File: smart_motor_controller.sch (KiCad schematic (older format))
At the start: 42 parts, among them J10 USB_B_Micro, J101 Breakout, J102 I2C_CONN, J103 CAN_CONN, J104 Debug, J9 Input 12V, Q101 FDD6685, SW102 SW_NRST, SW103 SW_NRST, U2 STM32F405RGT6, U3 USBLC6-2SC6

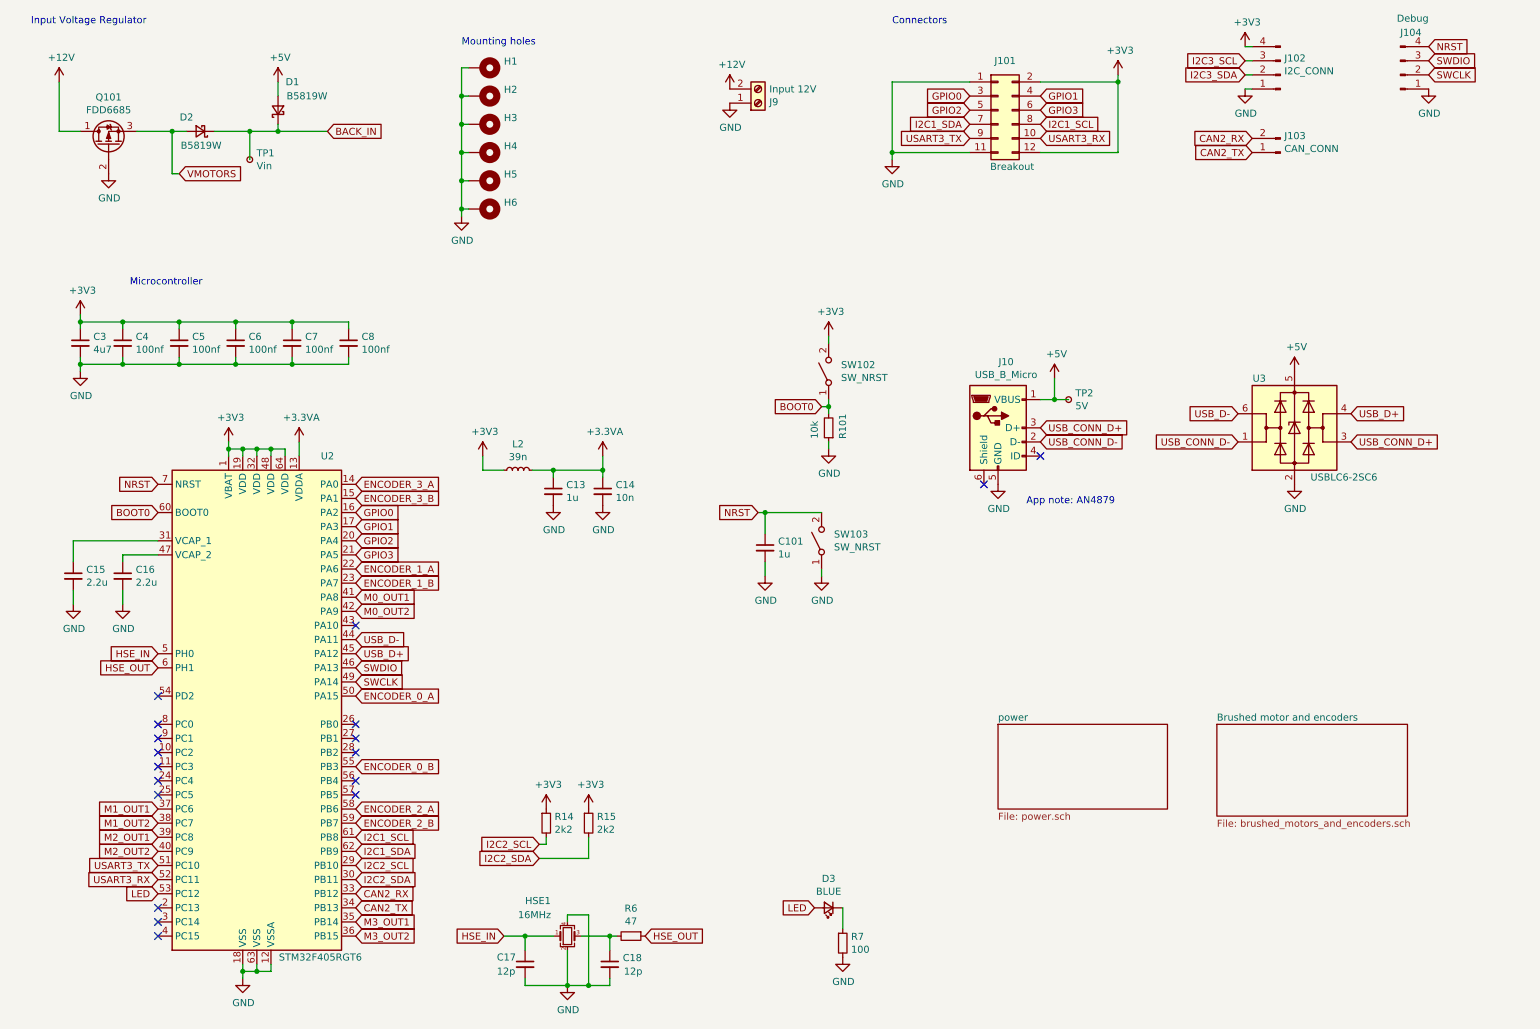
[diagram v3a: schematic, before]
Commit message: Additional changes
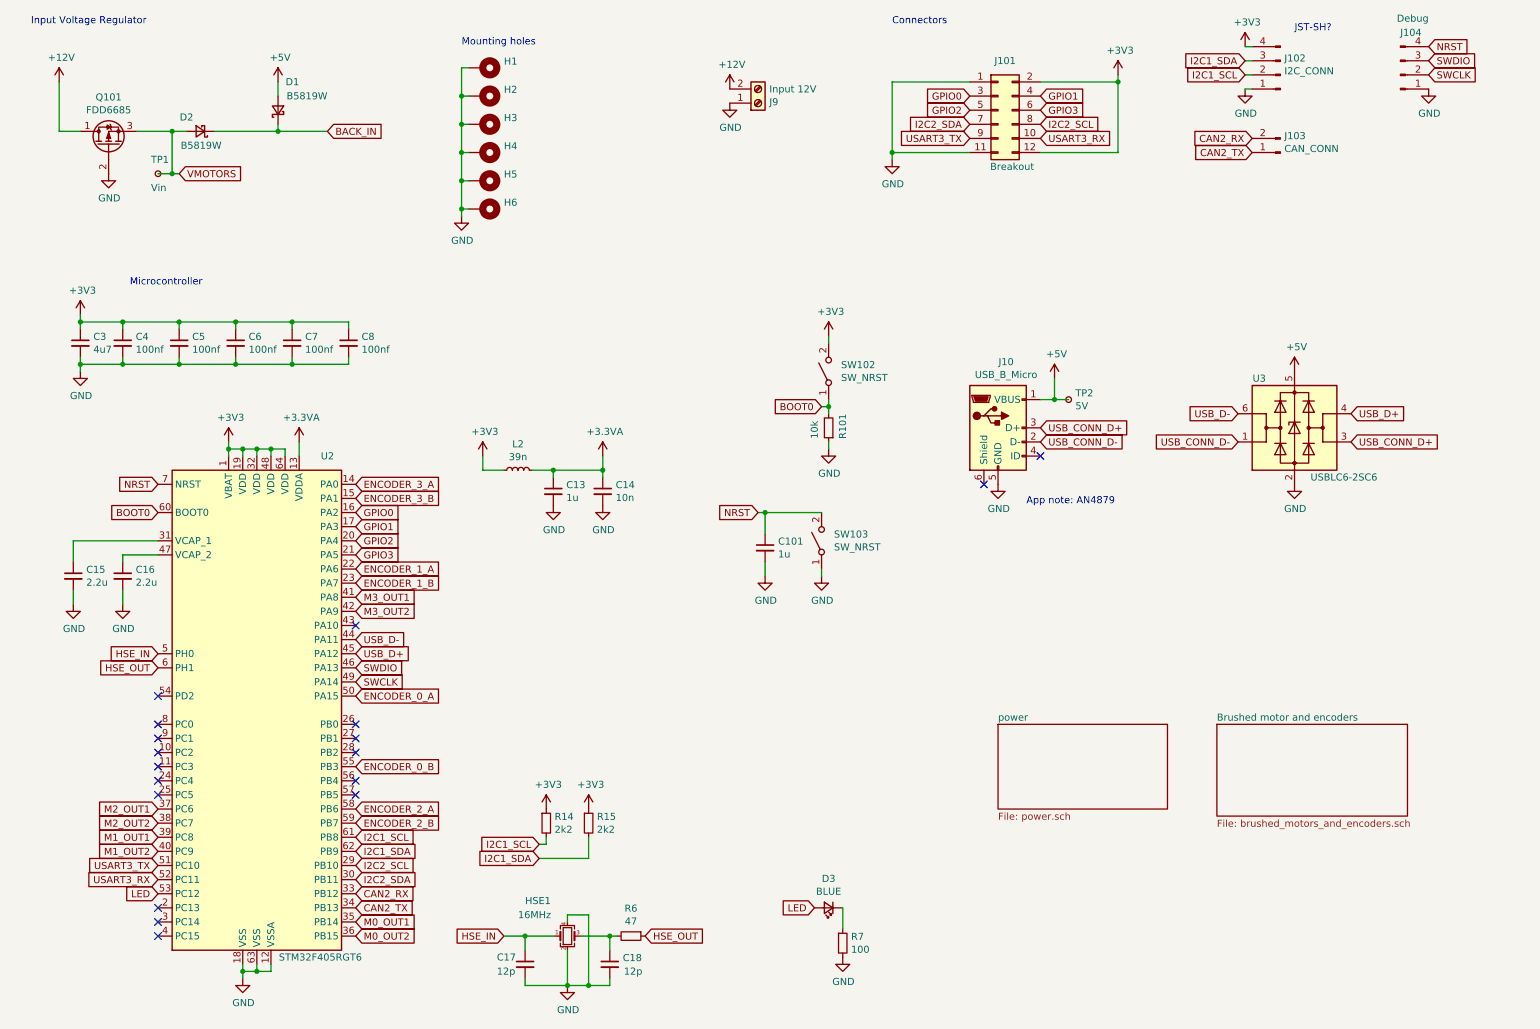
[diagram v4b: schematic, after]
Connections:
- net I2C3_SCL is gone; now on net I2C1_SDA: J102.3 (Pin_3)
- net I2C3_SDA is gone; now on net I2C1_SCL: J102.2 (Pin_2)
- net BACK_IN: no longer TP1.1
- net I2C1_SCL: now also R14.2; no longer J101.8 (Pin_8)
- net I2C1_SDA: now also R15.2; no longer J101.7 (Pin_7)
- net I2C2_SCL: now also J101.8 (Pin_8); no longer R14.2
- net I2C2_SDA: now also J101.7 (Pin_7); no longer R15.2
- net M0_OUT1: now also U2.35 (PB14); no longer U2.41 (PA8)
- net M0_OUT2: now also U2.36 (PB15); no longer U2.42 (PA9)
- net M1_OUT1: now also U2.39 (PC8); no longer U2.37 (PC6)
- net M1_OUT2: now also U2.40 (PC9); no longer U2.38 (PC7)
- net M2_OUT1: now also U2.37 (PC6); no longer U2.39 (PC8)
- net M2_OUT2: now also U2.38 (PC7); no longer U2.40 (PC9)
- net M3_OUT1: now also U2.41 (PA8); no longer U2.35 (PB14)
- net M3_OUT2: now also U2.42 (PA9); no longer U2.36 (PB15)
- net VMOTORS: now also TP1.1
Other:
- note added: "JST-SH?"
- moved on the sheet: TP1
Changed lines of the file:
@@
 Text Notes 1300 2500 0    50   ~ 0
 Microcontroller
-Text GLabel 7750 1350 2    50   Input ~ 0
+Text GLabel 9200 1000 0    50   Input ~ 0
 I2C1_SCL
-Text GLabel 7250 1350 0    50   Input ~ 0
+Text GLabel 9200 900  0    50   Input ~ 0
 I2C1_SDA
 $Comp
@@
 $EndComp
 NoConn ~ 2900 5800
+Text GLabel 2900 7000 2    50   Input ~ 0
+M0_OUT1
+Text GLabel 2900 7100 2    50   Input ~ 0
+M0_OUT2
+Text GLabel 1500 6400 0    50   Input ~ 0
+M1_OUT1
+Text GLabel 1500 6500 0    50   Input ~ 0
+M1_OUT2
+Text GLabel 1500 6200 0    50   Input ~ 0
+M2_OUT1
+Text GLabel 1500 6300 0    50   Input ~ 0
+M2_OUT2
 Text GLabel 2900 4700 2    50   Input ~ 0
-M0_OUT1
+M3_OUT1
 Text GLabel 2900 4800 2    50   Input ~ 0
-M0_OUT2
-Text GLabel 1500 6200 0    50   Input ~ 0
-M1_OUT1
-Text GLabel 1500 6300 0    50   Input ~ 0
-M1_OUT2
-Text GLabel 1500 6400 0    50   Input ~ 0
-M2_OUT1
-Text GLabel 1500 6500 0    50   Input ~ 0
-M2_OUT2
-Text GLabel 2900 7000 2    50   Input ~ 0
-M3_OUT1
-Text GLabel 2900 7100 2    50   Input ~ 0
 M3_OUT2
 NoConn ~ 2900 4900
@@
 Text GLabel 9250 1550 0    50   Input ~ 0
 CAN2_TX
-Text GLabel 9200 900  0    50   Input ~ 0
-I2C3_SCL
-Text GLabel 9200 1000 0    50   Input ~ 0
-I2C3_SDA
+Text GLabel 7750 1350 2    50   Input ~ 0
+I2C2_SCL
+Text GLabel 7250 1350 0    50   Input ~ 0
+I2C2_SDA
 $Comp
 L power:+3V3 #PWR0104
@@
 	4200 6450 4250 6450
 Text GLabel 4200 6550 0    50   Input ~ 0
-I2C2_SDA
+I2C1_SDA
 Text GLabel 4200 6450 0    50   Input ~ 0
-I2C2_SCL
+I2C1_SCL
 $Comp
 L Device:R_Small R15
@@
 L Connector:TestPoint_Small TP1
 U 1 1 604A4E02
-P 2150 1600
-F 0 "TP1" H 2198 1646 50  0000 L CNN
-F 1 "Vin" H 2198 1555 50  0000 L CNN
-F 2 "TestPoint:TestPoint_Pad_D1.5mm" H 2350 1600 50  0001 C CNN
-F 3 "~" H 2350 1600 50  0001 C CNN
-	1    2150 1600
-	1    0    0    -1
-$EndComp
-Wire Wire Line
-	1900 1400 2150 1400
+P 1500 1700
+F 0 "TP1" H 1450 1800 50  0000 L CNN
+F 1 "Vin" H 1450 1600 50  0000 L CNN
+F 2 "TestPoint:TestPoint_Pad_D1.5mm" H 1700 1700 50  0001 C CNN
+F 3 "~" H 1700 1700 50  0001 C CNN
+	1    1500 1700
+	1    0    0    -1
+$EndComp
 Connection ~ 2350 1400
-Wire Wire Line
-	2150 1600 2150 1400
-Connection ~ 2150 1400
-Wire Wire Line
-	2150 1400 2350 1400
 Wire Wire Line
 	1350 1400 1600 1400
@@
 	1    0    0    -1
 $EndComp
-Text GLabel 2900 5900 2    50   Input ~ 0
-ENCODER_0_B
-Text GLabel 2900 5400 2    50   Input ~ 0
-ENCODER_0_A
-Text GLabel 2900 4600 2    50   Input ~ 0
-ENCODER_1_B
-Text GLabel 2900 6300 2    50   Input ~ 0
-ENCODER_2_B
-Text GLabel 2900 6200 2    50   Input ~ 0
-ENCODER_2_A
-Text GLabel 2900 4000 2    50   Input ~ 0
-ENCODER_3_B
-Text GLabel 2900 3900 2    50   Input ~ 0
-ENCODER_3_A
 Text GLabel 1500 6600 0    50   Input ~ 0
 USART3_TX
 Text GLabel 1500 6700 0    50   Input ~ 0
 USART3_RX
-Text GLabel 2900 4500 2    50   Input ~ 0
-ENCODER_1_A
 NoConn ~ 2900 6000
 NoConn ~ 2900 6100
@@
 Text GLabel 10500 900  2    50   Input ~ 0
 SWDIO
+Text GLabel 2900 6200 2    50   Input ~ 0
+ENCODER_2_A
+Text GLabel 2900 6300 2    50   Input ~ 0
+ENCODER_2_B
+Text GLabel 2900 4500 2    50   Input ~ 0
+ENCODER_1_A
+Text GLabel 2900 4600 2    50   Input ~ 0
+ENCODER_1_B
+Text GLabel 2900 4000 2    50   Input ~ 0
+ENCODER_3_B
+Text GLabel 2900 3900 2    50   Input ~ 0
+ENCODER_3_A
+Text GLabel 2900 5400 2    50   Input ~ 0
+ENCODER_0_A
+Text GLabel 2900 5900 2    50   Input ~ 0
+ENCODER_0_B
+Wire Wire Line
+	1500 1700 1600 1700
+Connection ~ 1600 1700
+Wire Wire Line
+	1900 1400 2350 1400
+Text Notes 9550 700  0    50   ~ 0
+JST-SH?
 $EndSCHEMATC

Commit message: Fixed issue with diodes
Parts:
- R7: LCSC Part # C25076 -> C22775
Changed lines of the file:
@@
 F 2 "Resistor_SMD:R_0603_1608Metric" H 6350 7150 50  0001 C CNN
 F 3 "~" H 6350 7150 50  0001 C CNN
-F 4 "C25076" H 6350 7150 50  0001 C CNN "LCSC Part #"
+F 4 "C22775" H 6350 7150 50  0001 C CNN "LCSC Part #"
 	1    6350 7150
 	1    0    0    -1
